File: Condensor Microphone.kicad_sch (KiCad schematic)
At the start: 11 parts, among them U3 MAX9814

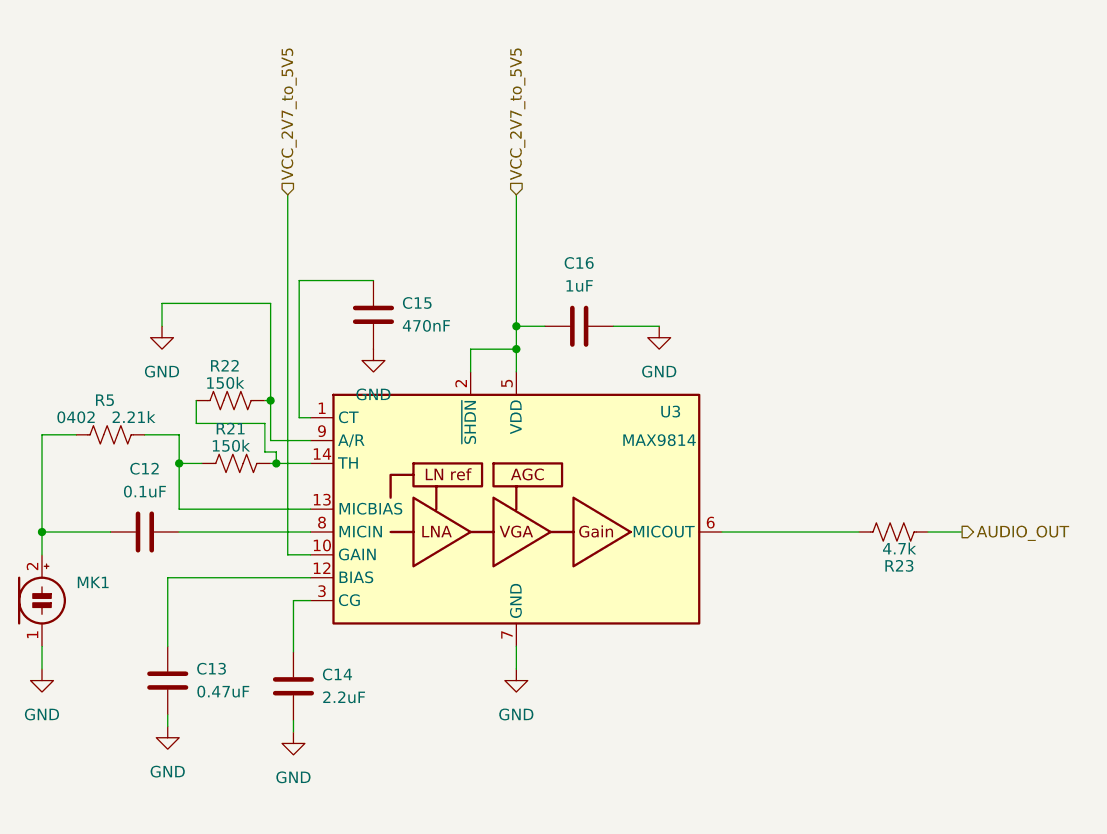
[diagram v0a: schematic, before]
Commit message: partially routed
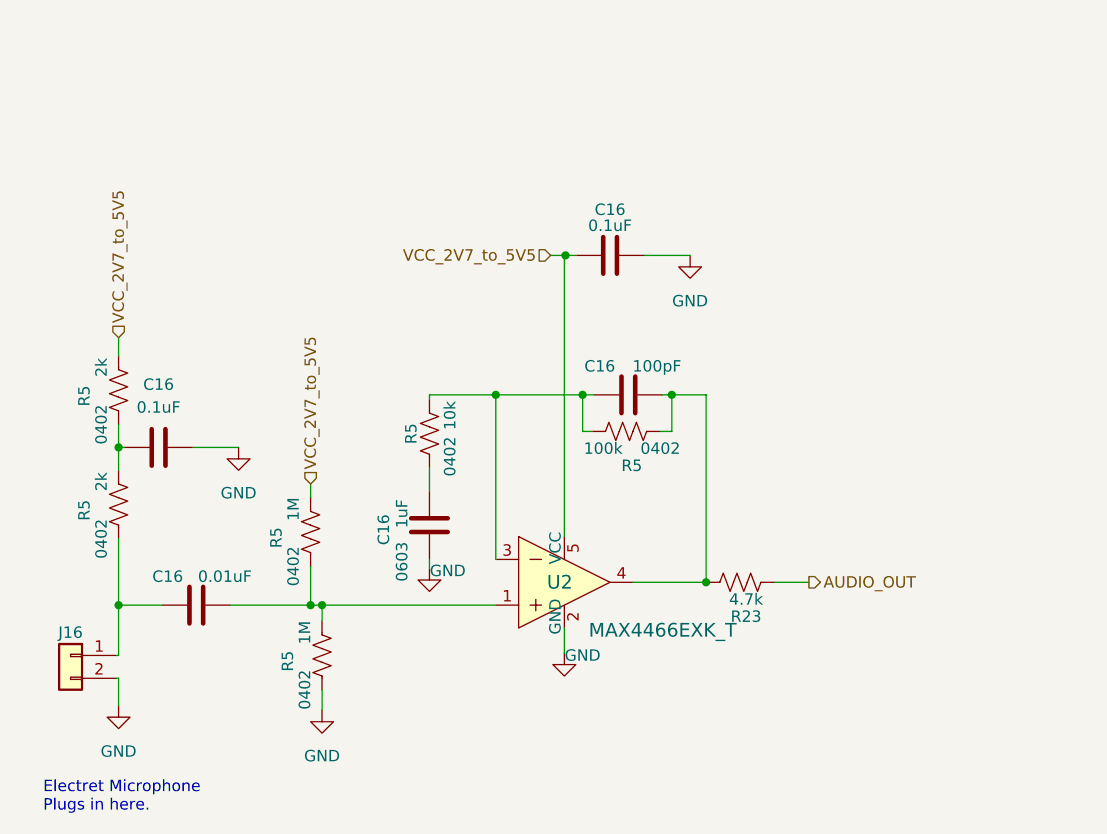
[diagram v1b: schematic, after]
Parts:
- removed C12: 0.1uF, Capacitor_SMD:C_0402_1005Metric, symbol Device:C
- removed C13: 0.47uF, Capacitor_SMD:C_0402_1005Metric, symbol Device:C
- removed C14: 2.2uF, Capacitor_SMD:C_0603_1608Metric, symbol Device:C
- removed C15: 470nF, Capacitor_SMD:C_0402_1005Metric, symbol Device:C
- removed C16: 1uF, Capacitor_SMD:C_0402_1005Metric, symbol Device:C
- removed MK1: Microphone_Condenser, microphone:MIC_AOM-6545_PUI, symbol Device:Microphone_Condenser
- removed R21, R22: 150k, Resistor_SMD:R_0402_1005Metric, symbol Device:R_US
- removed R5: 2.21k, Resistor_SMD:R_0402_1005Metric, symbol Device:R_US
- removed U3: MAX9814, Package_DFN_QFN:DFN-14-1EP_3x3mm_P0.4mm_EP1.78x2.35mm, symbol Amplifier_Audio:MAX9814
- added C16: 1uF, Capacitor_SMD:C_0603_1608Metric, symbol Device:C
- added C16 (x2): 0.1uF, Capacitor_SMD:C_0402_1005Metric, symbol Device:C
- added C16: 0.01uF, Capacitor_SMD:C_0402_1005Metric, symbol Device:C
- added C16: 100pF, Capacitor_SMD:C_0402_1005Metric, symbol Device:C
- added J16: Conn_01x02, 1x2FemaleVertical:PinHeader_1x02_P2.54mm_VerticalFemale, symbol 4ms_Connector:Conn_01x02
- added R5 (x2): 1M, Resistor_SMD:R_0402_1005Metric, symbol Device:R_US
- added R5: 10k, Resistor_SMD:R_0402_1005Metric, symbol Device:R_US
- added R5: 100k, Resistor_SMD:R_0402_1005Metric, symbol Device:R_US
- added R5 (x2): 2k, Resistor_SMD:R_0402_1005Metric, symbol Device:R_US
- added U2: MAX4466EXK_T, digikey-footprints:SOT-353, symbol dk_Linear-Amplifiers-Audio:MAX4466EXK_T
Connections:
- net GND: now also C16.1, C16.2, C16.2, J16.2 (Pin_2), R5.1, U2.2 (GND)
- net VCC_2V7_to_5V5: now also C16.1, R5.2, R5.2, U2.5 (VCC)
- net at R23.2: now also C16.2, R5.1, U2.4
- new net: C16.2, R5.1
- new net: C16.1, J16.1 (Pin_1), R5.1
- new net: C16.2, R5.1, R5.2, U2.1
- new net: C16.1, R5.2, R5.2, U2.3
- new net: C16.1, R5.1, R5.2
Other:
- note added: "Electret Microphone Plugs in here."
